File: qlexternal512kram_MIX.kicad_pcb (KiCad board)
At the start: 2 copper layers, 97.8 x 41.3 mm, 15 parts, among them J1 QL_SLOT_DIN41612_CARD, J2 QL_SLOT_DIN41612_CARD, U1 HM628512BLFP-7, U2 GAL16V8B-25QP, U3 LM1117-5.0

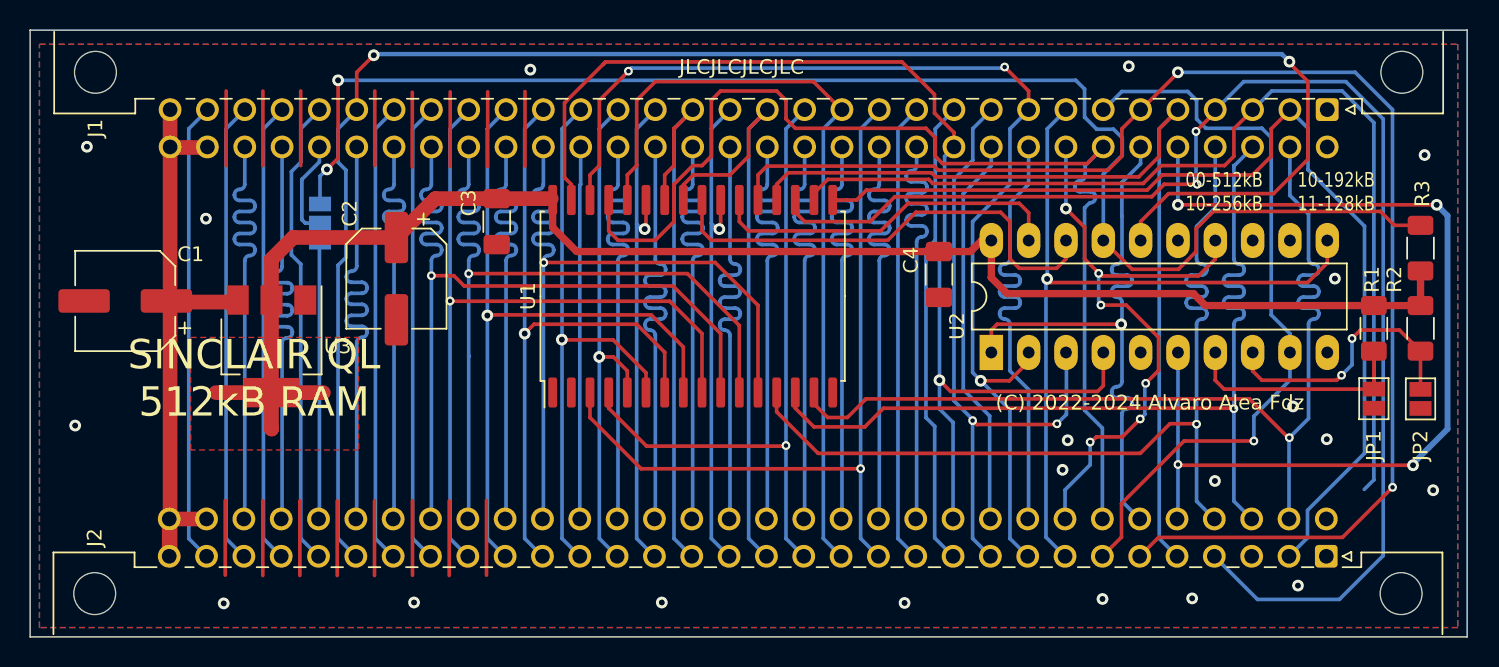
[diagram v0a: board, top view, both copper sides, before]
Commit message: version pre-release 1
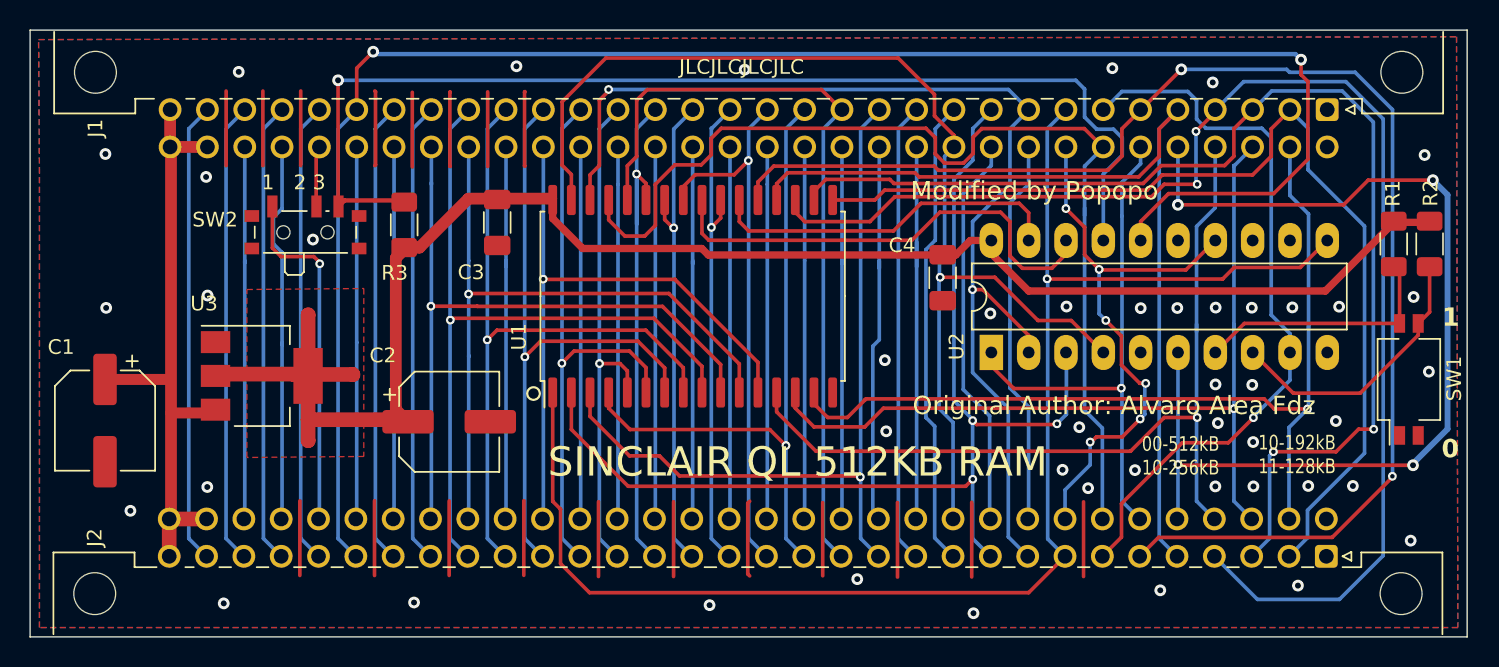
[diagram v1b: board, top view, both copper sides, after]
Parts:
- removed JP1, JP2: Jumper_2_Open, Jumper:SolderJumper-2_P1.3mm_Open_Pad1.0x1.5mm
- removed JP3: Jumper_3_Open, Jumper:SolderJumper-3_P1.3mm_Open_Pad1.0x1.5mm
- added REF**: KiCad-Logo2_5mm_SilkScreen, Symbol:KiCad-Logo2_5mm_SilkScreen, B.Cu at (101.8, 67.3)
- added REF**: Symbol_Attention_Triangle_8x7mm_Copper, Symbol:Symbol_Attention_Triangle_8x7mm_Copper, B.Cu at (115.6, 77.7)
- added REF**: OSHW-Logo_5.7x6mm_SilkScreen, Symbol:OSHW-Logo_5.7x6mm_SilkScreen, B.Cu at (101.7, 74.0)
- added SW1: SW_DIP_x02, Button_Switch_SMD:SW_DIP_SPSTx02_Slide_KingTek_DSHP02TS_W7.62mm_P1.27mm, F.Cu at (186.6, 76.1)
- added SW2: SW_SPDT, Button_Switch_SMD:SW_SPDT_PCM12, F.Cu at (111.5, 65.8)
- moved R3 69.2 mm to (118.3, 65.6)
- moved C2 10.4 mm to (121.3, 79.0), turned to 0 degrees
- moved C1 8.26 mm to (97.9, 78.9), turned to -90 degrees
- moved R1 5.90 mm to (185.6, 66.9)
- moved R2 5.78 mm to (188.0, 66.9)
- moved U3 2.12 mm to (108.6, 75.9), turned to 0 degrees
- moved C4 0.33 mm to (154.9, 69.2)
- moved C3 0.07 mm to (124.6, 65.5)
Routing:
- net /A18: track 52.7 -> 99.6 mm
- net /A16: track 43.4 -> 75.0 mm, vias 2 -> 3
- net Net-(SW2-C): track 97.9 -> 78.0 mm, vias 2 -> 1
- net GND: track 81.3 -> 96.6 mm, vias 20 -> 46
- net /D4: track 68.4 -> 79.3 mm, vias 0 -> 2
- net /A0: track 53.1 -> 44.3 mm
- net /A1: track 55.9 -> 47.7 mm
- net /A2: track 56.7 -> 48.7 mm
- net VCC: track 107.2 -> 114.6 mm
- net /VSYNC: track 31.4 -> 25.3 mm
- net /FC2: track 31.4 -> 25.3 mm
- net /GREEN: track 31.4 -> 25.3 mm
- net /IPL0: track 31.4 -> 25.3 mm
- net /VPA: track 31.4 -> 25.3 mm
- net /FC1: track 31.4 -> 25.3 mm
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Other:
- board text added: "0"
- board text added: "1"
- board text added: "1 2 3"
- board text added: "NOTE SW2: 1-2 Default Position 2-3 For use as +256Kb with Alvaro's Trump Card Install the +256K expansion after Alvaro's Trump Card"
- board text added: "Original Author: Alvaro Alea Fdz"
- board text added: "REV.1"
- board text added: "SINCLAIR QL 512KB RAM"
- board text added: "WARNING: Use it under your own risk. Combining this card with others without a proper Switches configuration may result in damage for your QL. Install it only with QL unplugged from power."
- board text removed: "(C) 2022-2024 Alvaro Alea Fdz"
- board text removed: "REV.3"
- board text removed: "SINCLAIR QL 512kB RAM"
